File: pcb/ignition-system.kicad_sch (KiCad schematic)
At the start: 11 parts, among them J1 IEC_60320_C14_Receptacle, J3 Conn_01x02, K1 FINDER-40.41, Q1 2N3904, SW1 SW_SPST, SW2 SW_Push

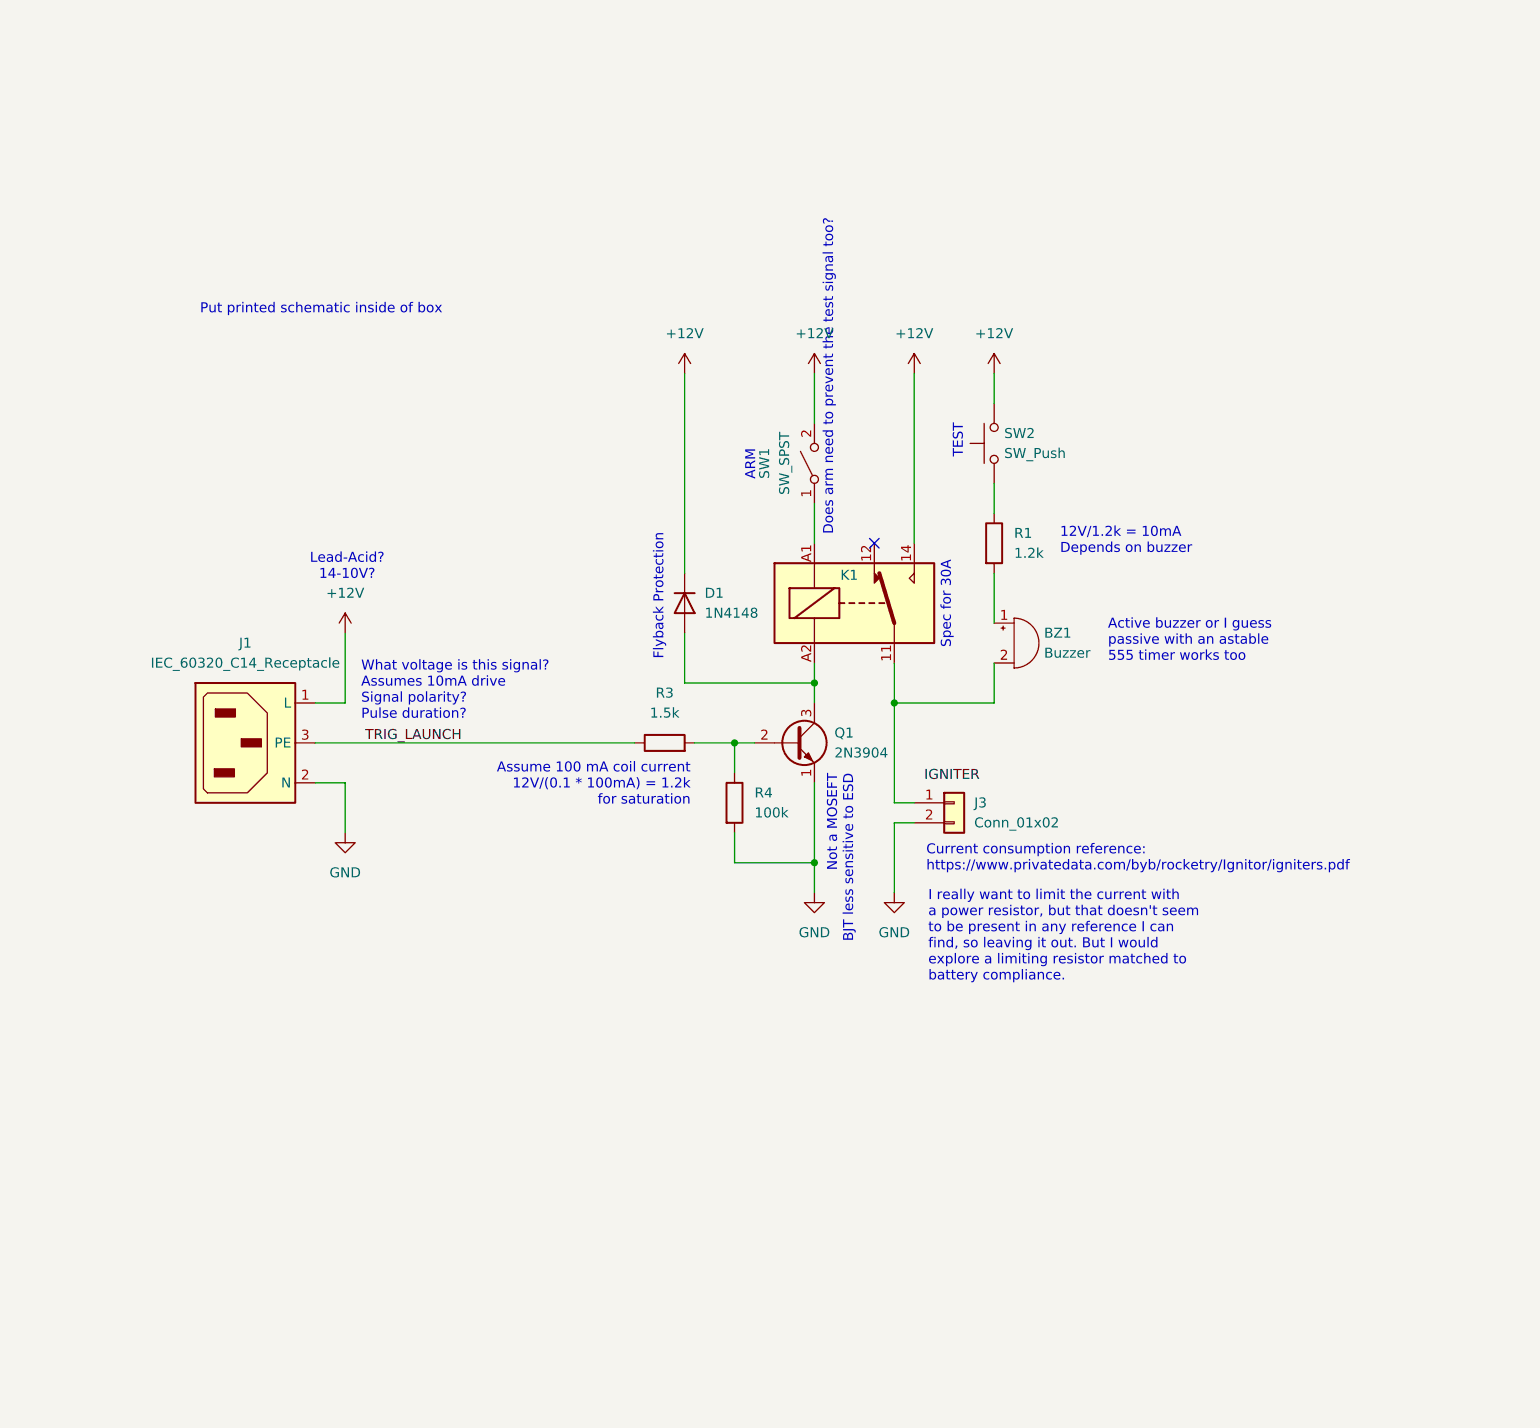
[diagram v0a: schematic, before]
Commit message: Update sch
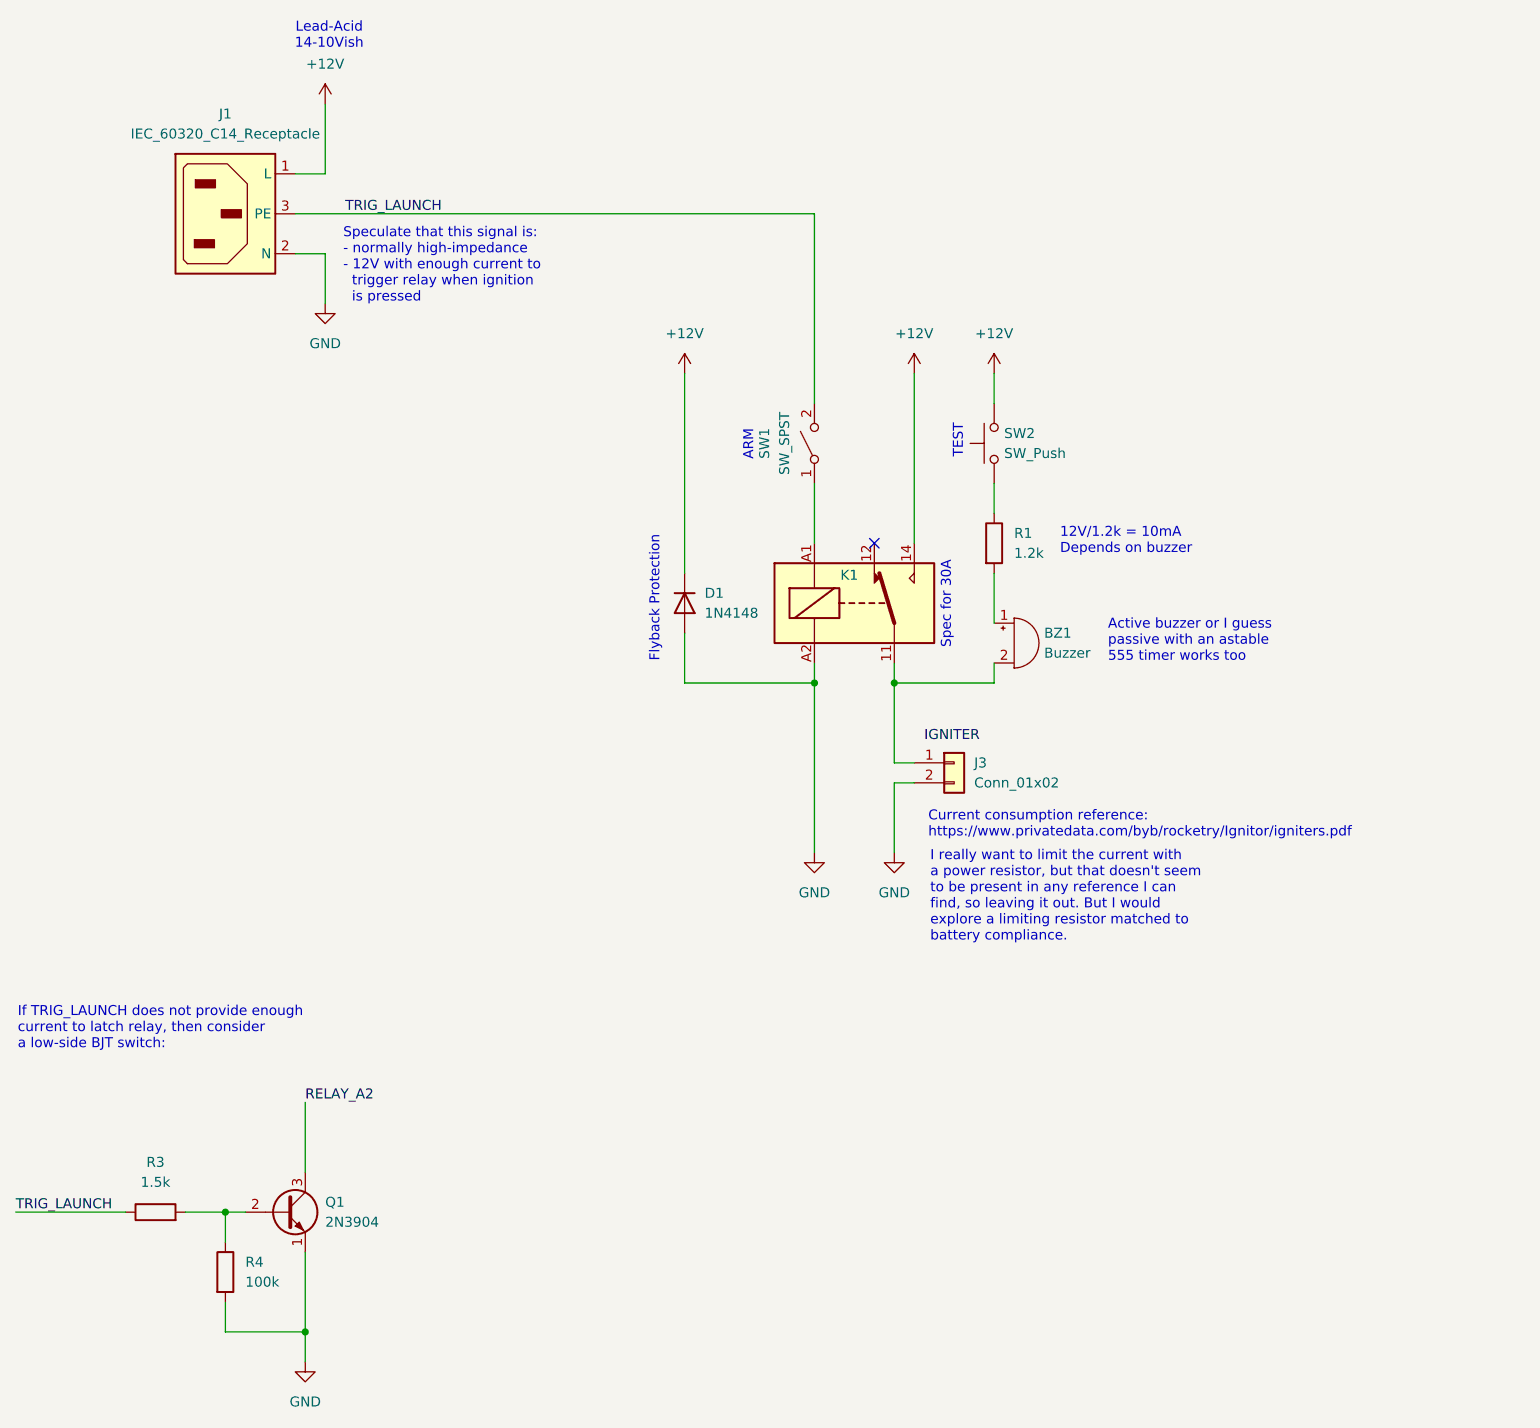
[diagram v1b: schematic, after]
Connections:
- net +12V: no longer SW1.2 (B)
- net GND: now also D1.2 (A), K1.A2
- net TRIG_LAUNCH: now also SW1.2 (B)
- new net RELAY_A2: Q1.3 (C)
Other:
- note added: "If TRIG_LAUNCH does not provide enough current to latch relay, then consider a low-side BJT switch:"
- note added: "Lead-Acid 14-10Vish"
- note added: "Speculate that this signal is: - normally high-impedance - 12V with enough current to trigger relay when ignition is pressed"
- note removed: "Assume 100 mA coil current 12V/(0.1 * 100mA) = 1.2k for saturation"
- note removed: "Does arm need to prevent the test signal too?"
- note removed: "Lead-Acid? 14-10V?"
- note removed: "Not a MOSEFT BJT less sensitive to ESD"
- note removed: "Put printed schematic inside of box"
- note removed: "What voltage is this signal? Assumes 10mA drive Signal polarity? Pulse duration?"
- moved on the sheet: J1, J3, Q1, R3, R4, SW1
